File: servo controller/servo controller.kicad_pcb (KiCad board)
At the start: 4 copper layers, 30 parts, among them J1 Conn_02x05_Odd_Even, J2 Conn_01x03, J3 Conn_01x03, J4 Conn_01x03, Q1 BC337, Q2 BC337, Q3 BC337, Q4 BC337, Q5 BC337, Q6 BC337, U2 L7805

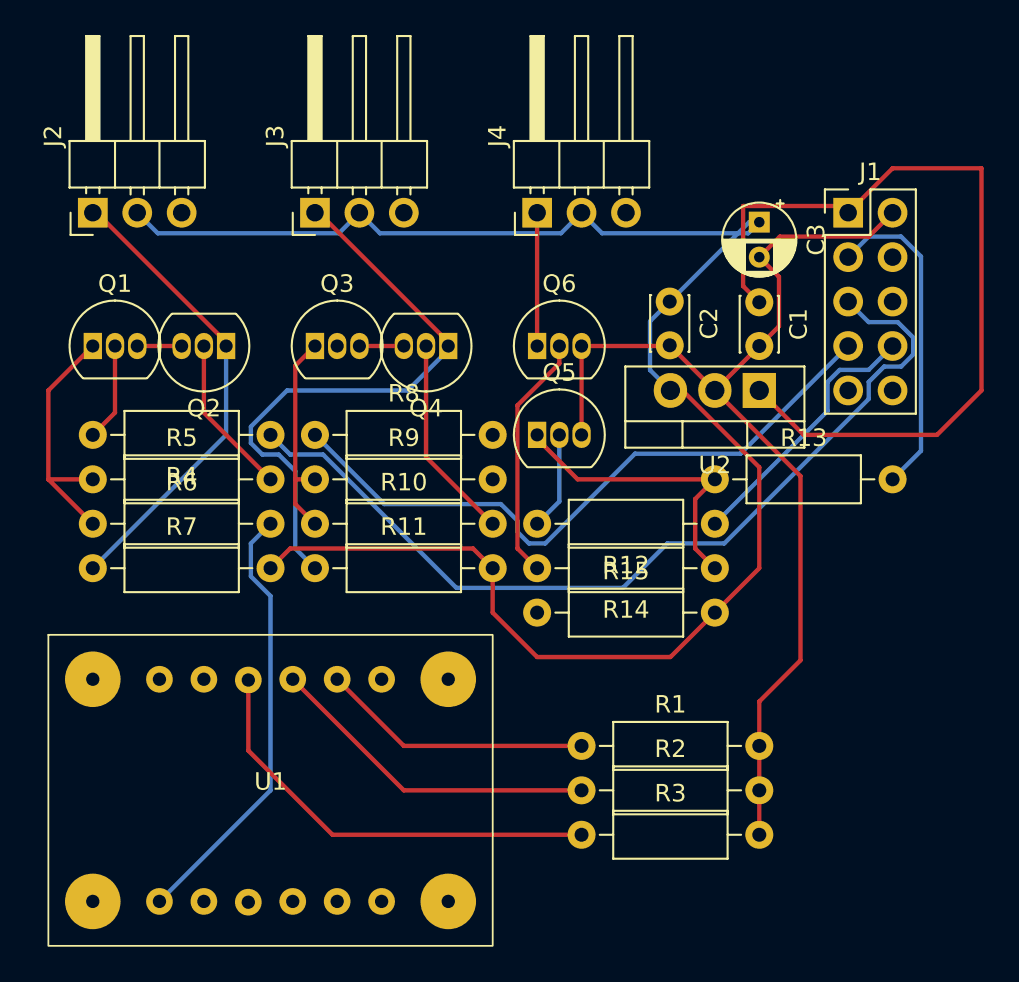
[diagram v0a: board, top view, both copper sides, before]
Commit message: Updates to flex parts and controller
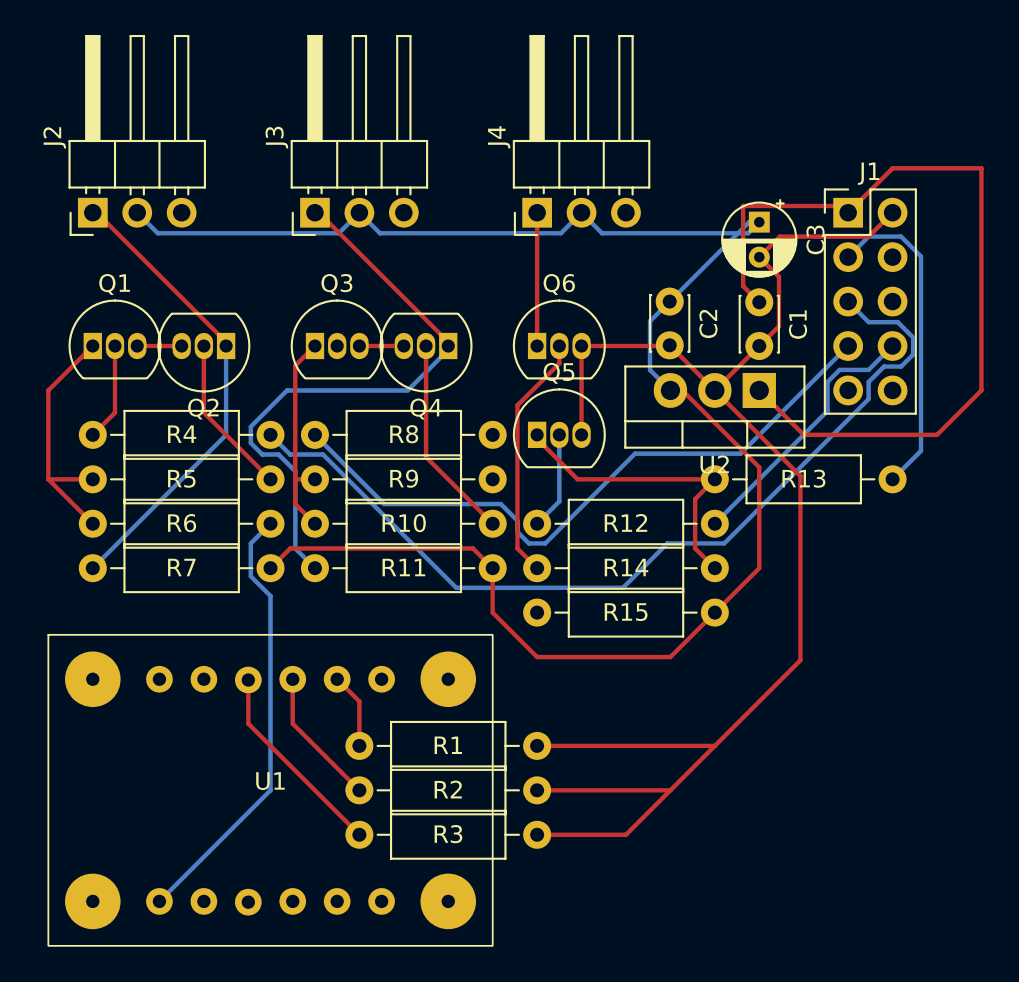
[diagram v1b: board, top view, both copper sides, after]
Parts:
- moved R1 12.7 mm to (96.5, 81.3)
- moved R2 12.7 mm to (96.5, 83.8)
- moved R3 12.7 mm to (96.5, 86.4)
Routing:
- net GND: track 122.5 -> 148.6 mm
- net Net-(J4-Pin_3): track 81.7 -> 68.1 mm
- net Net-(J3-Pin_3): track 51.9 -> 40.7 mm
- net Net-(J2-Pin_3): track 45.9 -> 34.7 mm
